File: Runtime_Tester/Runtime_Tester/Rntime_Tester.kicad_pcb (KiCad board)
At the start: 2 copper layers, 50.3 x 19.7 mm, 26 parts, among them IC1 RT9193-33GB, J1 USB1061-XX-X-X_REVA, J2 Conn_01x04_Pin, SW1 Reset, SW2 Continue, U1 STM32F103C8Tx, U2 CAT24C256, Y1 Crystal

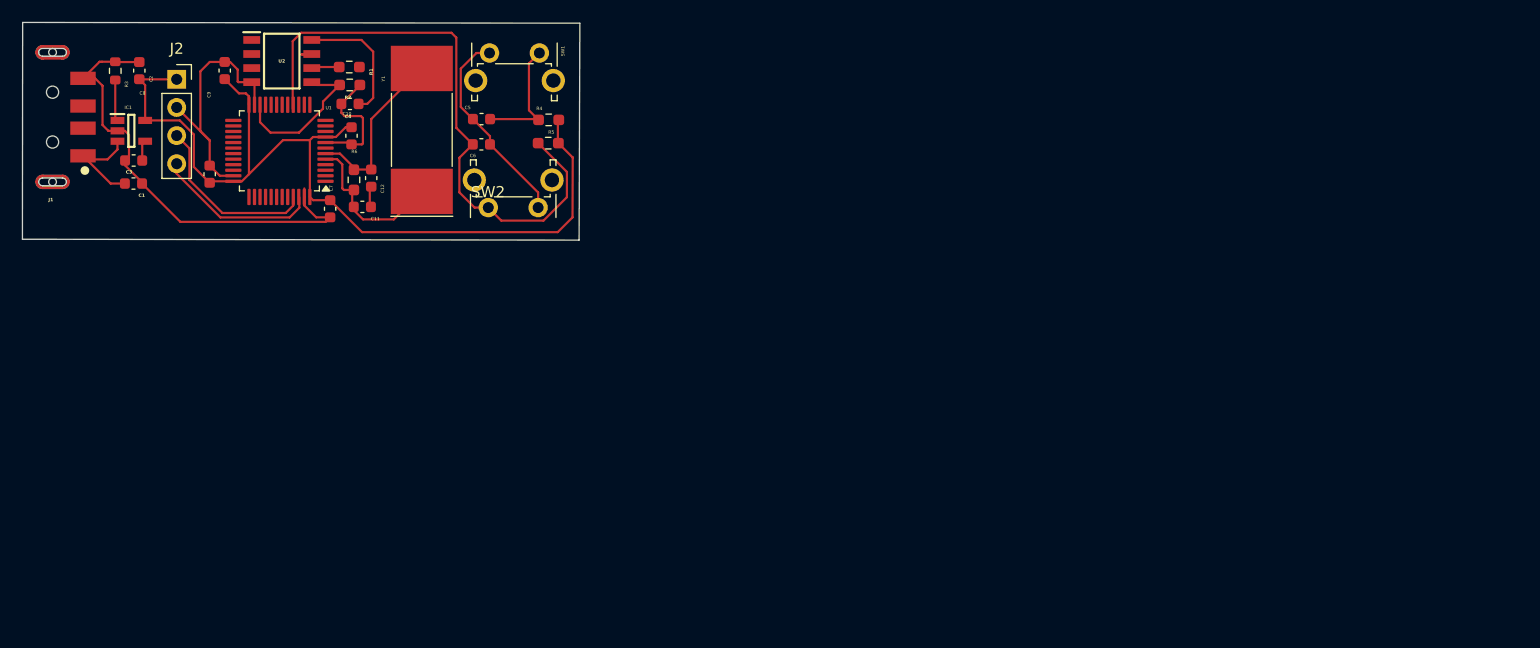
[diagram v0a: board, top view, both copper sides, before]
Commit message: pcb routing
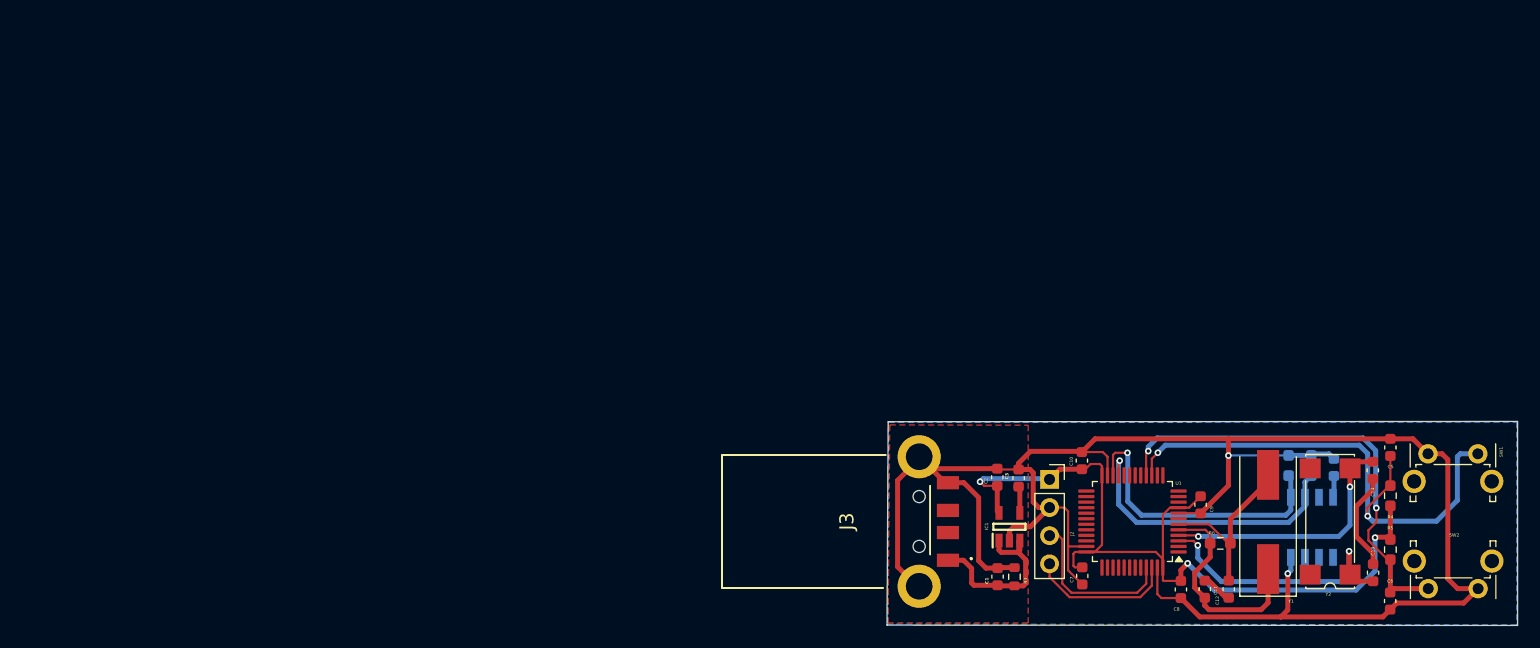
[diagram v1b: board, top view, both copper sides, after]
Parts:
- removed J1: USB1061-XX-X-X_REVA, USBA_Male:USBA_Male
- added C13: 20pF, Capacitor_SMD:C_0603_1608Metric, F.Cu at (167.3, 99.9)
- added C14: 20pF, Capacitor_SMD:C_0603_1608Metric, F.Cu at (167.3, 90.7)
- added J3: 48037-2100, USBA_Male_connector:480372100, F.Cu at (117.9, 95.3)
- added Y2: Crystal, Crystal:Crystal_SMD_SeikoEpson_MA406-4Pin_11.7x4.0mm, F.Cu at (163.4, 95.3)
- C10, C8: value 100 nF -> 100nF
- C11, C12: value C_Small -> 20pF
- C4, R1, R2, U2: moved to B.Cu
- J2: value Conn_01x04_Pin -> Oled display
- R6: value R -> 1M
- Y1: footprint Crystal:Crystal_SMD_SeikoEpson_MA505-2Pin_12.7x5.1mm -> Crystal:Crystal_SMD_HC49-SD
- moved U2 102.1 mm to (161.8, 95.8), turned to 90 degrees
- moved C9 96.5 mm to (151.7, 93.8), turned to -90 degrees
- moved C8 95.4 mm to (149.9, 101.4), turned to -90 degrees
- moved C4 94.7 mm to (163.8, 90.4), turned to 90 degrees
- moved R1 94.0 mm to (161.7, 90.3), turned to -90 degrees
- moved R3 93.2 mm to (134.9, 100.3)
- moved SW1 92.2 mm to (172.2, 89.2)
- moved C6 91.8 mm to (168.8, 102.5), turned to -90 degrees
- moved SW2 91.6 mm to (176.8, 101.4)
- moved R2 91.5 mm to (159.7, 90.3), turned to -90 degrees
- moved C5 87.3 mm to (168.9, 88.6), turned to 90 degrees
- moved IC1 87.0 mm to (134.4, 95.8), turned to 90 degrees
- moved J2 86.7 mm to (138.1, 91.5)
- moved C12 85.9 mm to (154.3, 101.4)
- moved C2 85.7 mm to (133.4, 91.3)
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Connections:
- U1 pad 3: unconnected-(U1-PC14-Pad3) -> /PC14
- U1 pad 4: unconnected-(U1-PC15-Pad4) -> /PC15
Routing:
- net GND: track 96.7 -> 179.9 mm, vias 0 -> 2
- net /Reset: track 11.8 -> 48.8 mm, vias 0 -> 2
- net /PC14: track 0.00 -> 24.5 mm, vias 0 -> 2
- net /EEPROM_SCL: track 2.51 -> 26.5 mm, vias 0 -> 1
- net /PC15: track 0.00 -> 23.4 mm, vias 0 -> 2
- net /EEPROM_SDA: track 13.9 -> 26.3 mm, vias 0 -> 1
- net /Continue: track 54.1 -> 41.8 mm, vias 0 -> 2
- net +3V3: track 11.7 -> 1.95 mm
- net Net-(C13-Pad2): track 0.00 -> 8.93 mm
- net +3.3V: track 82.6 -> 75.6 mm, vias 0 -> 3
- net /OSC_IN: track 14.6 -> 21.6 mm
- net +5V: track 11.8 -> 16.8 mm
- net /Oled_SDA: track 14.9 -> 13.3 mm
- net /Oled_SCL: track 16.4 -> 15.0 mm
- net unconnected-(U2-WP-Pad7): track 1.37 -> 0.00 mm
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- added copper zone on B.Cu, net GND
- added copper zone on F.Cu, net GND
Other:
- board size 50.3 x 19.7 mm -> 56.9 x 18.4 mm
